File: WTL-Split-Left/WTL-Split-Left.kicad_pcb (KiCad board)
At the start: 2 copper layers, 142.9 x 77.8 mm, 51 parts, among them J1 MJ-4PP-9, U1 ProMicro

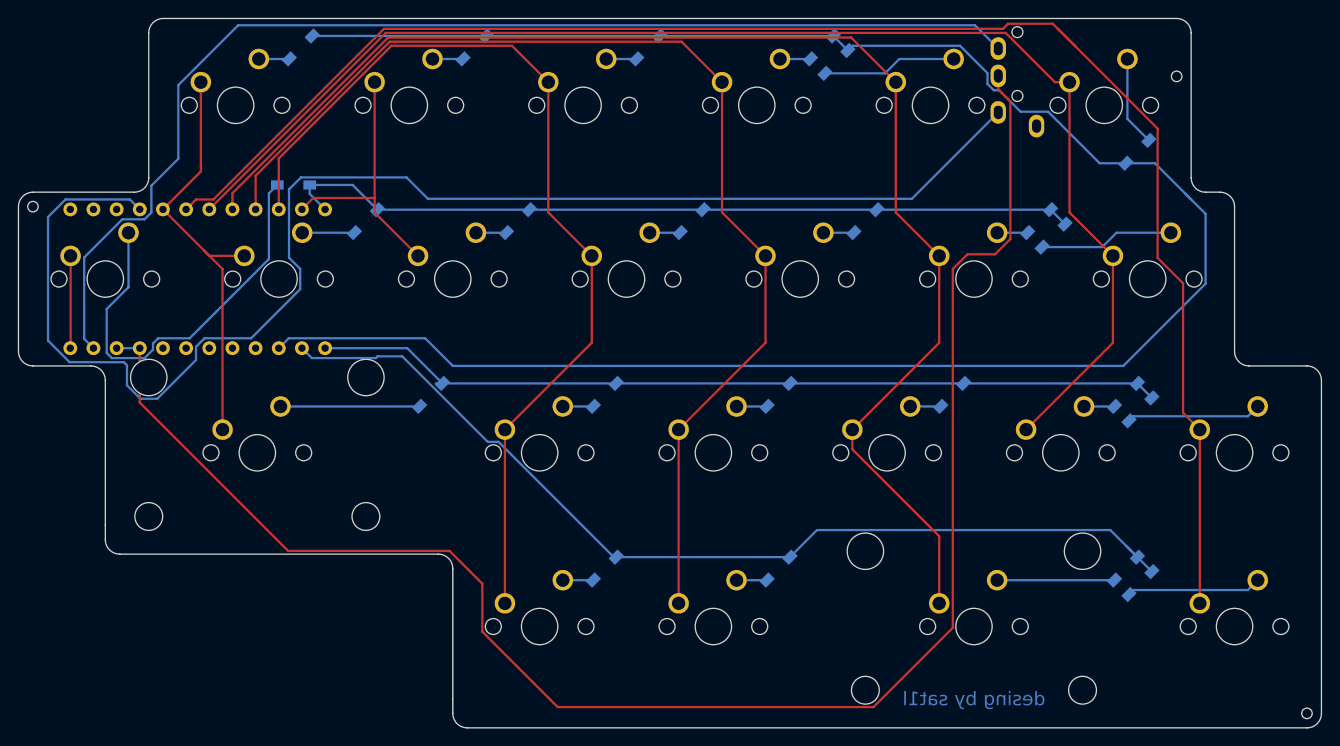
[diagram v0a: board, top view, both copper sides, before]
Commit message: tf i did?
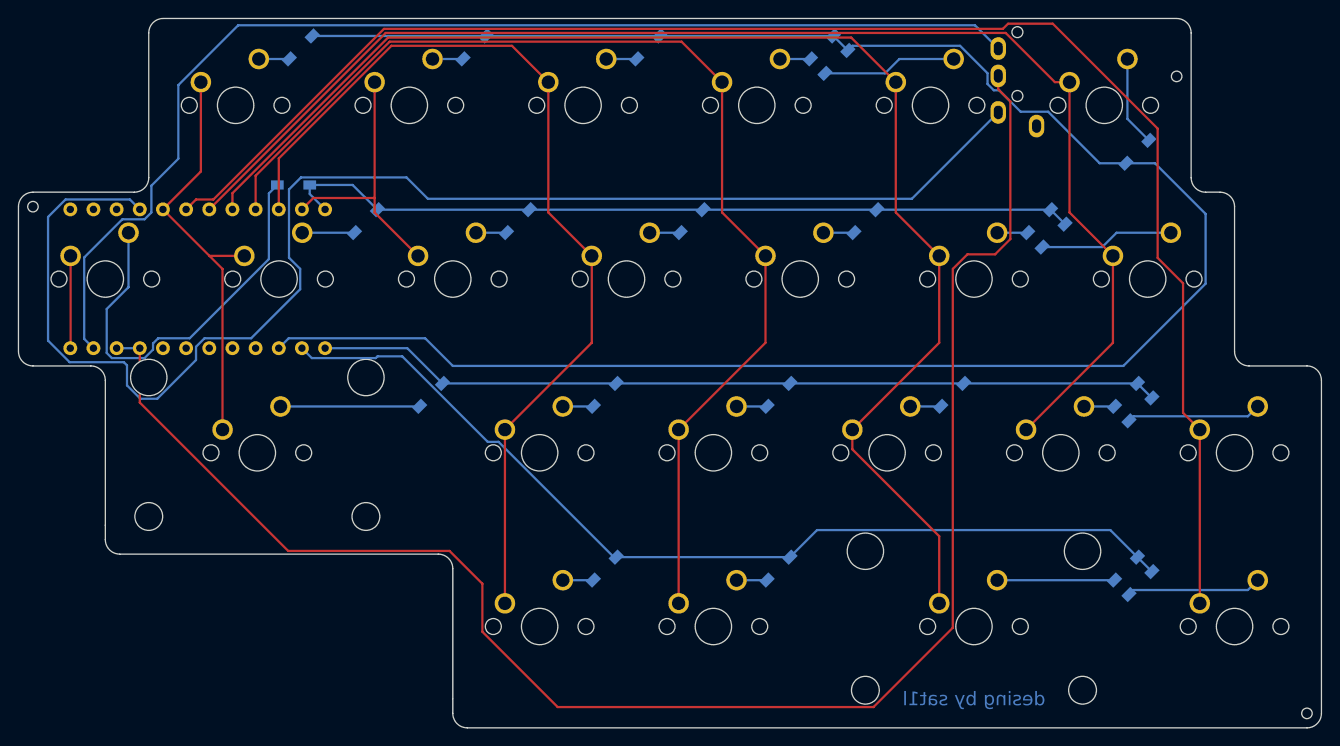
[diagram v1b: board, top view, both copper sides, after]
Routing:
- net col8: track 176.5 -> 173.7 mm
- net row4: track 107.1 -> 106.0 mm
- net row1: track 222.9 -> 221.9 mm
- net col2: track 47.2 -> 46.4 mm
- net row3: track 93.7 -> 92.9 mm
- net GND: track 184.4 -> 183.6 mm
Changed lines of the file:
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@@
   (segment (start 121.44375 61.11875) (end 194.974752 61.11875) (width 0.25) (layer "B.Cu") (net 2))
   (segment (start 192.375248 38.89375) (end 195.2625 38.89375) (width 0.25) (layer "B.Cu") (net 2))
-  (segment (start 202.40625 42.8625) (end 201.719751 42.176001) (width 0.25) (layer "B.Cu") (net 2))
+  (segment (start 198.4375 38.89375) (end 203.99375 44.45) (width 0.25) (layer "B.Cu") (net 2))
   (segment (start 181.362258 30.89376) (end 183.712238 33.24374) (width 0.25) (layer "B.Cu") (net 2))
-  (segment (start 203.99375 44.45) (end 198.4375 38.89375) (width 0.25) (layer "B.Cu") (net 2))
   (segment (start 183.712238 33.24374) (end 186.725238 33.24374) (width 0.25) (layer "B.Cu") (net 2))
   (segment (start 163.180115 24.938635) (end 164.767615 26.526135) (width 0.25) (layer "B.Cu") (net 2))
@@
   (segment (start 102.5525 65.56375) (end 117.7925 65.56375) (width 0.25) (layer "B.Cu") (net 16))
   (segment (start 196.517615 63.038635) (end 198.105115 64.626135) (width 0.25) (layer "B.Cu") (net 17))
-  (segment (start 120.317615 63.038635) (end 119.566386 63.038635) (width 0.25) (layer "B.Cu") (net 17))
   (segment (start 120.317615 63.038635) (end 116.45238 59.1734) (width 0.25) (layer "B.Cu") (net 17))
   (segment (start 116.45238 59.1734) (end 107.442 59.1734) (width 0.25) (layer "B.Cu") (net 17))
@@
   (segment (start 125.273145 69.443749) (end 126.464751 69.443749) (width 0.25) (layer "B.Cu") (net 24))
   (segment (start 104.902 59.1734) (end 105.989001 60.260401) (width 0.25) (layer "B.Cu") (net 24))
-  (segment (start 196.12074 81.69176) (end 196.517615 82.088635) (width 0.25) (layer "B.Cu") (net 24))
+  (segment (start 193.548829 79.119849) (end 196.517615 82.088635) (width 0.25) (layer "B.Cu") (net 24))
   (segment (start 158.417615 82.088635) (end 161.386401 79.119849) (width 0.25) (layer "B.Cu") (net 24))
   (segment (start 113.186927 60.069849) (end 115.899245 60.069849) (width 0.25) (layer "B.Cu") (net 24))
@@
   (segment (start 112.996375 60.260401) (end 113.186927 60.069849) (width 0.25) (layer "B.Cu") (net 24))
   (segment (start 126.464751 69.443749) (end 139.109637 82.088635) (width 0.25) (layer "B.Cu") (net 24))
-  (segment (start 193.548829 79.119849) (end 196.12074 81.69176) (width 0.25) (layer "B.Cu") (net 24))
-  (segment (start 195.288729 80.859749) (end 196.12074 81.69176) (width 0.25) (layer "B.Cu") (net 24))
   (segment (start 161.386401 79.119849) (end 193.548829 79.119849) (width 0.25) (layer "B.Cu") (net 24))
   (segment (start 115.899245 60.069849) (end 125.273145 69.443749) (width 0.25) (layer "B.Cu") (net 24))
@@
   (segment (start 178.702597 23.765097) (end 181.25625 26.31875) (width 0.25) (layer "B.Cu") (net 30))
   (segment (start 88.392212 44.29195) (end 88.392212 41.35519) (width 0.25) (layer "B.Cu") (net 30))
-  (segment (start 94.1943 48.4857) (end 94.76235 49.05375) (width 0.25) (layer "F.Cu") (net 31))
   (segment (start 93.82125 39.79415) (end 89.662 43.9534) (width 0.25) (layer "F.Cu") (net 31))
   (segment (start 96.2025 68.10375) (end 96.195489 68.096739) (width 0.25) (layer "F.Cu") (net 31))
   (segment (start 96.195489 68.096739) (end 96.195489 50.486889) (width 0.25) (layer "F.Cu") (net 31))
-  (segment (start 93.82125 38.883888) (end 93.82125 39.79415) (width 0.25) (layer "F.Cu") (net 31))
-  (segment (start 89.662 43.9534) (end 94.1943 48.4857) (width 0.25) (layer "F.Cu") (net 31))
-  (segment (start 96.195489 50.486889) (end 94.1943 48.4857) (width 0.25) (layer "F.Cu") (net 31))
+  (segment (start 93.82125 30.00375) (end 93.82125 39.79415) (width 0.25) (layer "F.Cu") (net 31))
+  (segment (start 89.662 43.9534) (end 96.195489 50.486889) (width 0.25) (layer "F.Cu") (net 31))
   (segment (start 94.76235 49.05375) (end 98.58375 49.05375) (width 0.25) (layer "F.Cu") (net 31))
-  (segment (start 93.82125 30.00375) (end 93.82125 38.883888) (width 0.25) (layer "F.Cu") (net 31))
   (segment (start 112.87125 30.00375) (end 112.87125 42.70375) (width 0.25) (layer "F.Cu") (net 32))
   (segment (start 104.902 43.9534) (end 106.15165 42.70375) (width 0.25) (layer "F.Cu") (net 32))
@@
   (segment (start 95.192591 42.866399) (end 113.90275 24.15624) (width 0.25) (layer "F.Cu") (net 38))
   (segment (start 198.733749 35.092251) (end 198.733749 49.274849) (width 0.25) (layer "F.Cu") (net 38))
-  (segment (start 187.797738 24.15624) (end 189.770749 26.129251) (width 0.25) (layer "F.Cu") (net 38))
+  (segment (start 187.235247 23.593749) (end 198.733749 35.092251) (width 0.25) (layer "F.Cu") (net 38))
   (segment (start 182.331241 23.593749) (end 187.235247 23.593749) (width 0.25) (layer "F.Cu") (net 38))
   (segment (start 201.523749 52.064849) (end 201.523749 66.268749) (width 0.25) (layer "F.Cu") (net 38))
@@
   (segment (start 201.523749 66.268749) (end 203.35875 68.10375) (width 0.25) (layer "F.Cu") (net 38))
   (segment (start 181.76875 24.15624) (end 182.331241 23.593749) (width 0.25) (layer "F.Cu") (net 38))
-  (segment (start 187.235247 23.593749) (end 189.770749 26.129251) (width 0.25) (layer "F.Cu") (net 38))
-  (segment (start 189.770749 26.129251) (end 198.733749 35.092251) (width 0.25) (layer "F.Cu") (net 38))
   (segment (start 103.390238 81.40624) (end 121.09374 81.40624) (width 0.25) (layer "F.Cu") (net 47))
   (segment (start 180.912651 48.880851) (end 182.583751 47.209751) (width 0.25) (layer "F.Cu") (net 47))
@@
   (segment (start 124.688749 85.001249) (end 124.688749 90.269751) (width 0.25) (layer "F.Cu") (net 47))
   (segment (start 181.25625 30.787752) (end 181.25625 29.31875) (width 0.25) (layer "F.Cu") (net 47))
-  (segment (start 181.76875 29.83125) (end 181.25625 29.31875) (width 0.25) (layer "F.Cu") (net 47))
   (segment (start 87.122 59.1734) (end 87.122 65.138002) (width 0.25) (layer "F.Cu") (net 47))
   (segment (start 176.274849 50.480677) (end 177.874675 48.880851) (width 0.25) (layer "F.Cu") (net 47))
